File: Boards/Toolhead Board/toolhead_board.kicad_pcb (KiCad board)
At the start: 2 copper layers, 52 x 39.4 mm, 29 parts, among them J1 Molex 502386-0470, J10 Molex 502386-0370, J2 Molex 213228-1810, J3 Molex 502386-0370, J4 Molex 502386-0370, J5 Conn_02x04_Odd_Even, J6 Molex 502386-0470, J7 Molex 502386-0270, J8 Molex 502386-0370, J9 Molex 43650-0210, U1 HX717, U2 ST490ADBR

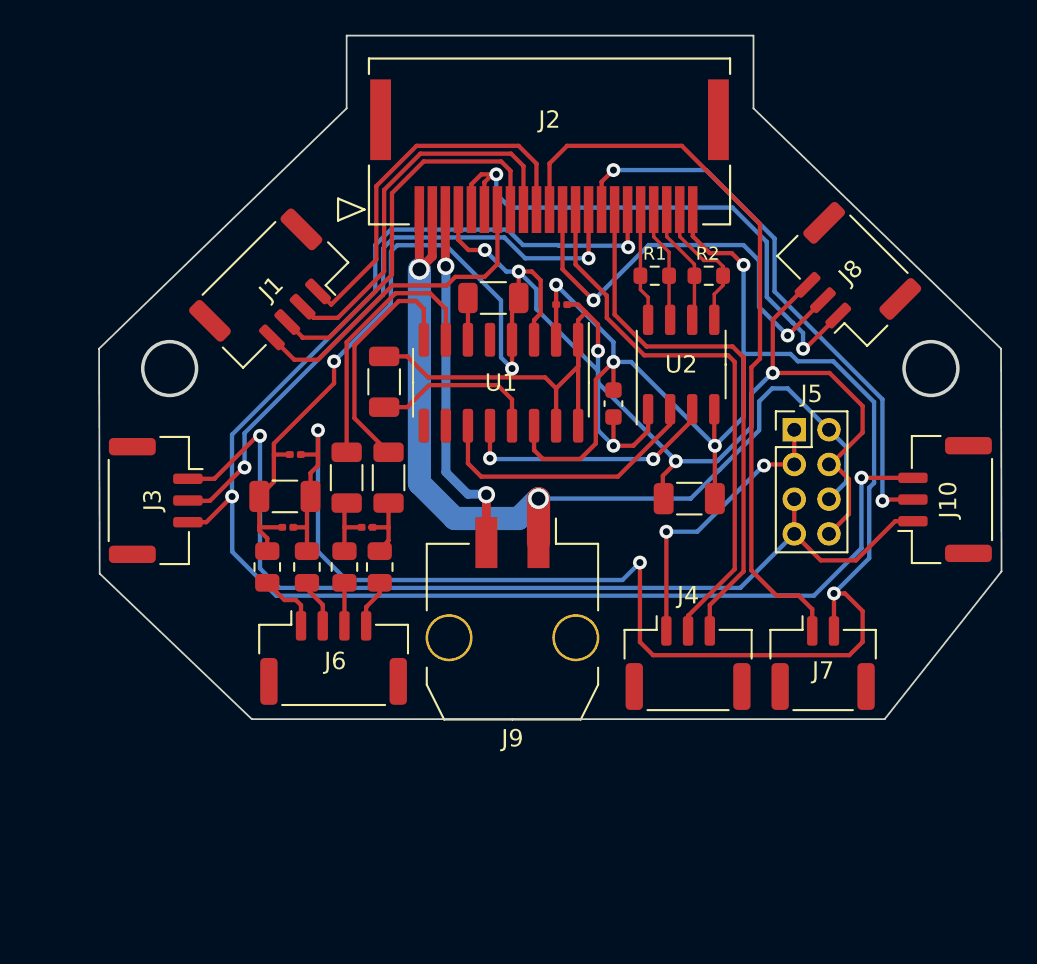
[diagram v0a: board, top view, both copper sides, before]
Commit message: 4 layer board
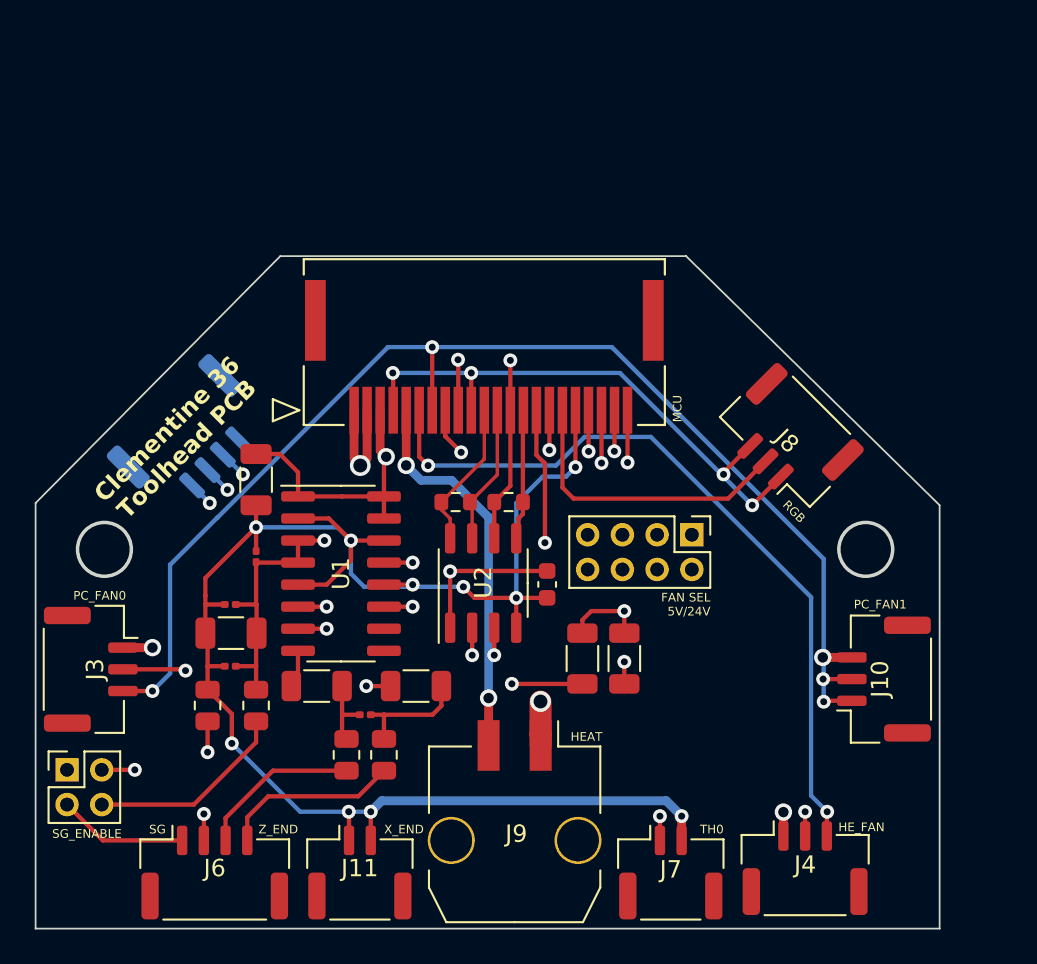
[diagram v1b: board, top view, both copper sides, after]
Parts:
- added J11: Molex 502386-0270, Connector_Molex:Molex_CLIK-Mate_502386-0270_1x02-1MP_P1.25mm_Horizontal, F.Cu at (97.3, 80.2)
- added J12: Conn_02x02_Odd_Even, Connector_PinHeader_2.00mm:PinHeader_2x02_P2.00mm_Vertical, F.Cu at (80.4, 74.3)
- J1: value Molex 502386-0470 -> Molex 502382-0470; footprint Connector_Molex:Molex_CLIK-Mate_502386-0470_1x04-1MP_P1.25mm_Horizontal -> Connector_Molex:Molex_CLIK-Mate_502382-0470_1x04-1MP_P1.25mm_Vertical; moved to B.Cu
- moved C6 25.0 mm to (91.3, 57.6), turned to 90 degrees
- moved C5 22.8 mm to (91.3, 62.0), turned to -90 degrees
- moved R5 21.4 mm to (110.1, 67.9), turned to 90 degrees
- moved R7 21.1 mm to (112.5, 67.9)
- moved R2 17.4 mm to (105.8, 58.9)
- moved R1 17.4 mm to (102.8, 58.9)
- moved U2 17.0 mm to (104.4, 63.5)
- moved J7 14.9 mm to (115.2, 80.2)
- moved U1 14.3 mm to (96.2, 63.0), turned to 0 degrees
- moved J6 14.1 mm to (88.9, 80.2)
- moved J4 13.6 mm to (122.9, 80.0)
- moved R3 12.7 mm to (94.8, 69.5), turned to 180 degrees
- moved R4 12.7 mm to (100.5, 69.5), turned to 180 degrees
- moved J2 12.2 mm to (96.9, 53.6)
- moved J9 11.7 mm to (106.2, 78.0)
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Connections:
- J1 pad 1: MOTOR_2B -> MOTOR_1A
- J1 pad 2: MOTOR_2A -> MOTOR_1B
- J1 pad 3: MOTOR_1B -> MOTOR_2A
- J1 pad 4: MOTOR_1A -> MOTOR_2B
- J10 pad 1: /PC_FAN_PWR -> PC_FAN_GND
- J10 pad 3: PC_FAN_GND -> /PC_FAN_PWR
- J2 pad 10: MOTOR_2B -> PC_FAN1_TACH
- J2 pad 11: TH0 -> SCK+
- J2 pad 12: RGB -> SCK-
- J2 pad 13: HE_FAN_TACH -> DATA-/Z_END
- J2 pad 14: PC_FAN0_TACH -> DATA+
- J2 pad 15: PC_FAN1_TACH -> XEND
- J2 pad 16: HE_FAN_GND -> TH0
- J2 pad 17: PC_FAN_GND -> RGB
- J2 pad 18: SCK+ -> GNDA
- J2 pad 19: SCK- -> MOTOR_1A
- J2 pad 20: DATA- -> MOTOR_1B
- J2 pad 21: DATA+ -> MOTOR_2A
- J2 pad 22: GNDA -> MOTOR_2B
- J2 pad 3: HE0 -> +5V
- J2 pad 4: +5V -> GND
- J2 pad 5: GND -> HE_GND
- J2 pad 6: GND -> HE_FAN_GND
- J2 pad 7: MOTOR_1A -> PC_FAN_GND
- J2 pad 8: MOTOR_1B -> HE_FAN_TACH
- J2 pad 9: MOTOR_2A -> PC_FAN0_TACH
- J6 pad 1: Net-(J6-Pin_1) -> Net-(J12-Pin_1)
- J9 pad 2: HE0 -> HE_GND
- L1 pad 1: Net-(J6-Pin_1) -> Net-(J12-Pin_4)
- L3 pad 1: Net-(J6-Pin_4) -> Net-(J6-Pin_3)
- L4 pad 1: Net-(J6-Pin_3) -> Net-(J6-Pin_4)
- R2 pad 1: DATA- -> DATA-/Z_END
- U2 pad 6: DATA- -> DATA-/Z_END
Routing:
- net DATA-/Z_END: track 0.00 -> 52.6 mm, vias 0 -> 2
- net /PC_FAN_PWR: track 55.7 -> 100.8 mm, vias 1 -> 2
- net XEND: track 0.00 -> 36.1 mm, vias 0 -> 2
- net GNDA: track 130.9 -> 94.8 mm, vias 7 -> 8
- net +5V: track 136.5 -> 102.9 mm, vias 8 -> 5
- net HE_GND: track 0.00 -> 22.3 mm, vias 0 -> 2
- net HE0: track 21.0 -> 0.00 mm, vias 2 -> 0
- net PC_FAN_GND: track 87.2 -> 70.7 mm
- net Net-(U1-S0): track 2.41 -> 18.2 mm, vias 0 -> 2
- net +24V: track 56.4 -> 43.3 mm
- net HE_FAN_GND: track 31.1 -> 44.1 mm, vias 0 -> 2
- net Net-(U1-S1): track 9.75 -> 22.5 mm, vias 0 -> 2
- net Net-(U1-INA+): track 14.0 -> 2.19 mm
- net Net-(J12-Pin_4): track 0.00 -> 11.6 mm
- net Net-(J12-Pin_1): track 0.00 -> 9.49 mm
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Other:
- board size 52 x 39.4 mm -> 52.1 x 38.7 mm
- copper layers 2 -> 4
- board text added: "Clementine 36 Toolhead PCB"
- board text added: "FAN SEL 5V/24V"
- board text added: "HEAT"
- board text added: "HE_FAN"
- board text added: "MCU"
- board text added: "MOTOR"
- board text added: "PC_FAN0"
- board text added: "PC_FAN1"
- board text added: "RGB"
- board text added: "SG"
- board text added: "SG_ENABLE"
- board text added: "TH0"
- board text added: "X_END"
- board text added: "Z_END"
